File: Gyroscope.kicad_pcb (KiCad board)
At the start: 2 copper layers, 5 parts, among them U1 IIS3DWB, U2 APS6404L-3SQRx-SN, U3 STM32G431C6Tx, U4 W25Q128JVS, U5 CR2013-MI2120

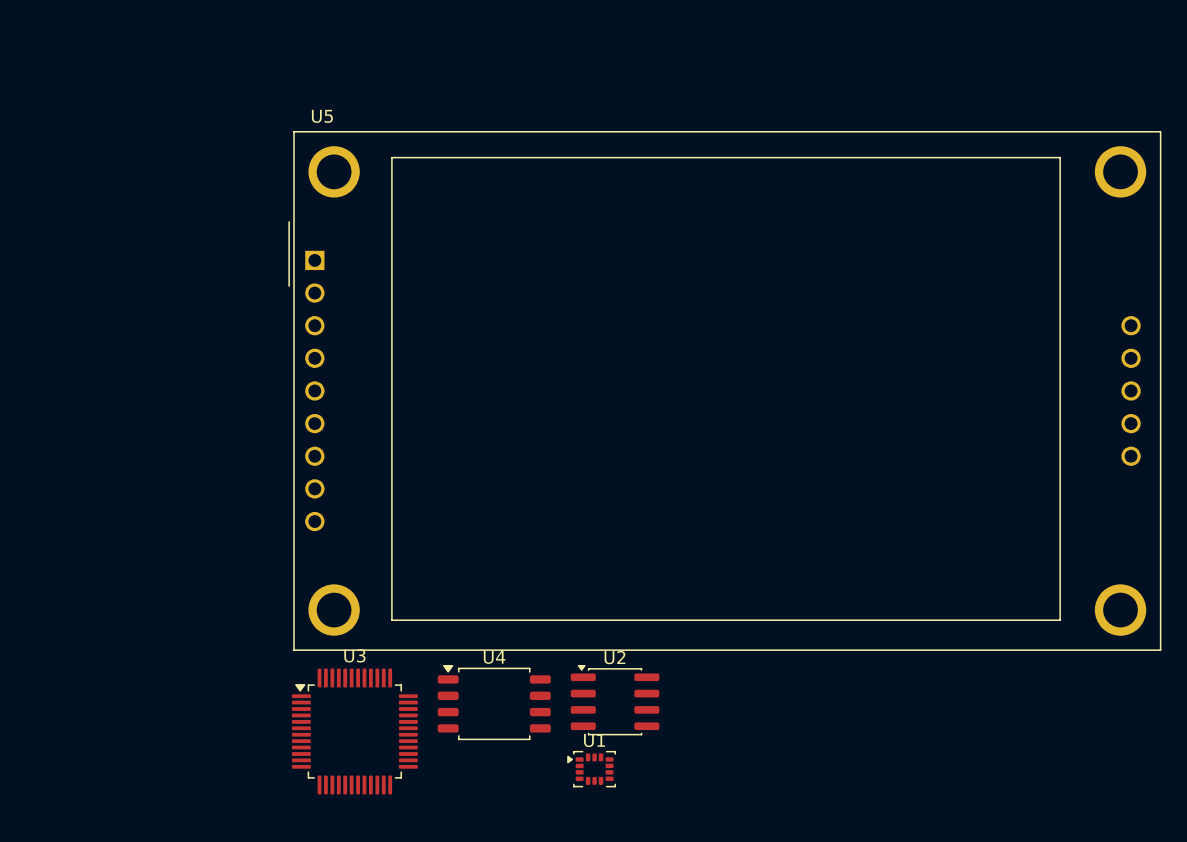
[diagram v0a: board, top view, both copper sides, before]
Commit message: refresh
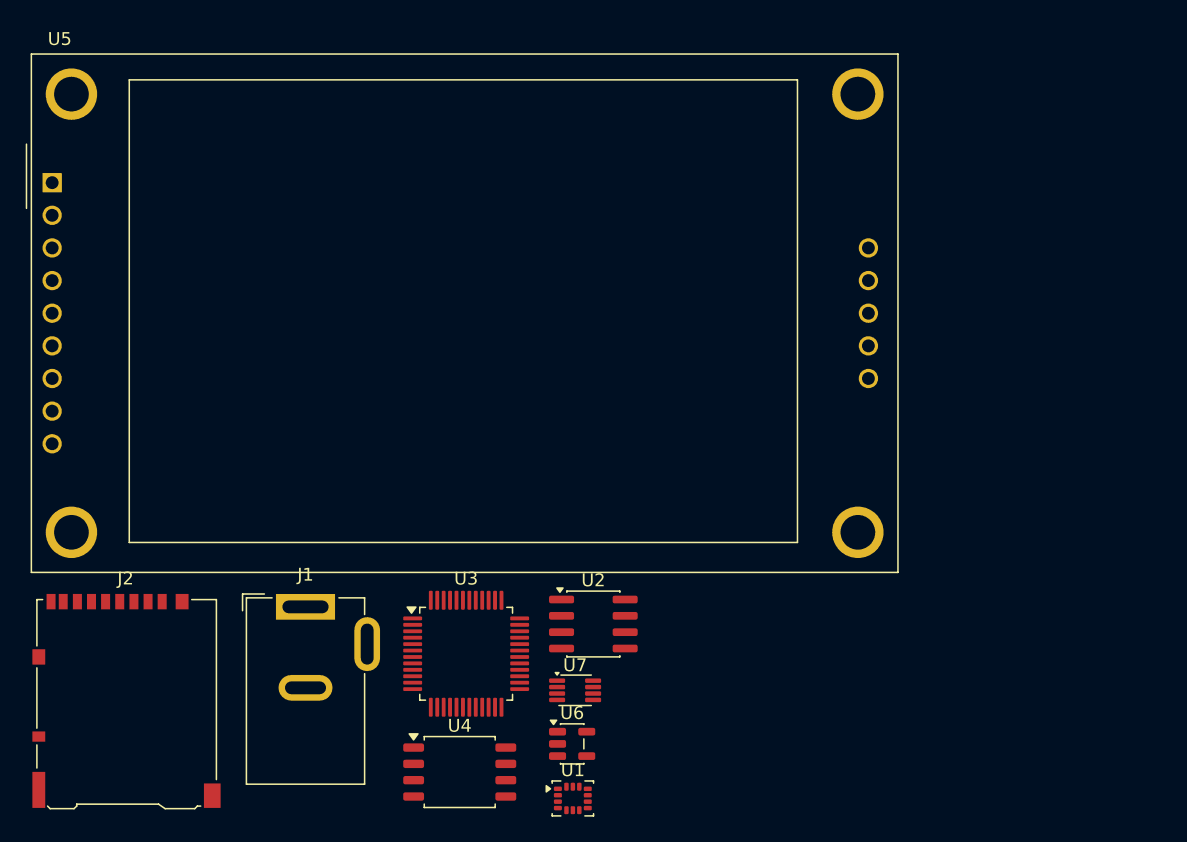
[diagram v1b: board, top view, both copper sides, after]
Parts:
- added J1: Barrel_Jack_Switch, Connector_BarrelJack:BarrelJack_GCT_DCJ200-10-A_Horizontal, F.Cu at (109.9, 96.2)
- added J2: Micro_SD_Card_Det2, Connector_Card:microSD_HC_Hirose_DM3AT-SF-PEJM5, F.Cu at (95.9, 103.5)
- added U6: AP2112K-3.3, Package_TO_SOT_SMD:SOT-23-5, F.Cu at (130.6, 106.9)
- added U7: 74LVC1G139, Package_SO:VSSOP-8_2.3x2mm_P0.5mm, F.Cu at (130.8, 102.7)
- moved U5 21.3 mm to (90.2, 63.2)
- moved U3 10.6 mm to (122.4, 99.9)
- moved U2 6.28 mm to (132.3, 97.6)
- moved U4 5.94 mm to (121.9, 109.1)
- moved U1 2.84 mm to (130.7, 111.1)
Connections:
- U1 pad 1: unconnected-(U1-SDO-Pad1) -> Net-(U1-SDO)
- U1 pad 12: unconnected-(U1-CS-Pad12) -> Net-(U1-CS)
- U1 pad 13: unconnected-(U1-SPC-Pad13) -> Net-(U1-SPC)
- U1 pad 14: unconnected-(U1-SDI-Pad14) -> Net-(U1-SDI)
- U1 pad 2: Net-(U1-GND-Pad2) -> GND
- U1 pad 3: Net-(U1-GND-Pad2) -> GND
- U1 pad 4: unconnected-(U1-INT1-Pad4) -> Net-(U1-INT1)
- U1 pad 5: unconnected-(U1-VDD_IO-Pad5) -> Net-(U1-VDD)
- U1 pad 6: Net-(U1-GND-Pad2) -> GND
- U1 pad 7: Net-(U1-GND-Pad2) -> GND
- U1 pad 8: unconnected-(U1-VDD-Pad8) -> Net-(U1-VDD)
- U1 pad 9: unconnected-(U1-INT2-Pad9) -> Net-(U1-INT2)
- U2 pad 1: unconnected-(U2-~{CE}-Pad1) -> Net-(U2-~{CE})
- U2 pad 2: unconnected-(U2-SO/SIO1-Pad2) -> Net-(U2-SO/SIO1)
- U2 pad 3: unconnected-(U2-SIO2-Pad3) -> Net-(U2-SIO2)
- U2 pad 4: unconnected-(U2-VSS-Pad4) -> GND
- U2 pad 5: unconnected-(U2-SI/SIO0-Pad5) -> Net-(U2-SI/SIO0)
- U2 pad 6: unconnected-(U2-SCLK-Pad6) -> Net-(U2-SCLK)
- U2 pad 7: unconnected-(U2-SIO3-Pad7) -> Net-(U2-SIO2)
- U2 pad 8: unconnected-(U2-VDD-Pad8) -> +3.3V
- U3 pad 1: unconnected-(U3-VBAT-Pad1) -> +3.3V
- U3 pad 12: unconnected-(U3-PA4-Pad12) -> Net-(U3-PA4)
- U3 pad 13: unconnected-(U3-PA5-Pad13) -> Net-(U3-PA5)
- U3 pad 14: unconnected-(U3-PA6-Pad14) -> Net-(U3-PA6)
- U3 pad 15: unconnected-(U3-PA7-Pad15) -> Net-(U3-PA7)
- U3 pad 19: unconnected-(U3-VSSA-Pad19) -> GND
- U3 pad 21: unconnected-(U3-VDDA-Pad21) -> Net-(U3-VDDA)
- U3 pad 23: Net-(U3-VSS-Pad23) -> GND
- U3 pad 24: unconnected-(U3-VDD-Pad24) -> +3.3V
- U3 pad 26: unconnected-(U3-PB12-Pad26) -> Net-(U2-~{CE})
- U3 pad 27: unconnected-(U3-PB13-Pad27) -> Net-(U2-SCLK)
- U3 pad 28: unconnected-(U3-PB14-Pad28) -> Net-(U2-SO/SIO1)
- U3 pad 29: unconnected-(U3-PB15-Pad29) -> Net-(U2-SI/SIO0)
- U3 pad 32: unconnected-(U3-PA10-Pad32) -> Net-(U3-PA10)
- U3 pad 33: unconnected-(U3-PA11-Pad33) -> Net-(U3-PA11)
- U3 pad 34: unconnected-(U3-PA12-Pad34) -> Net-(U3-PA12)
- U3 pad 35: Net-(U3-VSS-Pad23) -> GND
- U3 pad 36: unconnected-(U3-VDD-Pad36) -> +3.3V
- U3 pad 37: unconnected-(U3-PA13-Pad37) -> Net-(U1-INT2)
- U3 pad 38: unconnected-(U3-PA14-Pad38) -> Net-(U1-INT1)
- U3 pad 39: unconnected-(U3-PA15-Pad39) -> Net-(U1-CS)
- U3 pad 40: unconnected-(U3-PB3-Pad40) -> Net-(U1-SDO)
- U3 pad 41: unconnected-(U3-PB4-Pad41) -> Net-(U1-SDI)
- U3 pad 42: unconnected-(U3-PB5-Pad42) -> Net-(U1-SPC)
- U3 pad 47: Net-(U3-VSS-Pad23) -> GND
- U3 pad 48: unconnected-(U3-VDD-Pad48) -> +3.3V
- U4 pad 1: unconnected-(U4-~{CS}-Pad1) -> Net-(U3-PA4)
- U4 pad 2: unconnected-(U4-DO/IO_{1}-Pad2) -> Net-(U3-PA6)
- U4 pad 3: unconnected-(U4-~{WP}/IO_{2}-Pad3) -> Net-(U4-~{HOLD}/~{RESET}/IO_{3})
- U4 pad 4: unconnected-(U4-GND-Pad4) -> GND
- U4 pad 5: unconnected-(U4-DI/IO_{0}-Pad5) -> Net-(U3-PA7)
- U4 pad 6: unconnected-(U4-CLK-Pad6) -> Net-(U3-PA5)
- U4 pad 7: unconnected-(U4-~{HOLD}/~{RESET}/IO_{3}-Pad7) -> Net-(U4-~{HOLD}/~{RESET}/IO_{3})
- U4 pad 8: unconnected-(U4-VCC-Pad8) -> +3.3V
- U5 pad 2: unconnected-(U5-GND-Pad2) -> GND
- U5 pad 3: unconnected-(U5-~{CS}-Pad3) -> Net-(U3-PA12)
- U5 pad 6: unconnected-(U5-MOSI-Pad6) -> Net-(U3-PA11)
- U5 pad 9: unconnected-(U5-MISO-Pad9) -> Net-(U3-PA10)
